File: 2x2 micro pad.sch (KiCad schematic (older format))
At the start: 24 parts, among them SW1 SW_Push, U1 ATmega32U4-AU, Y1 16MHz

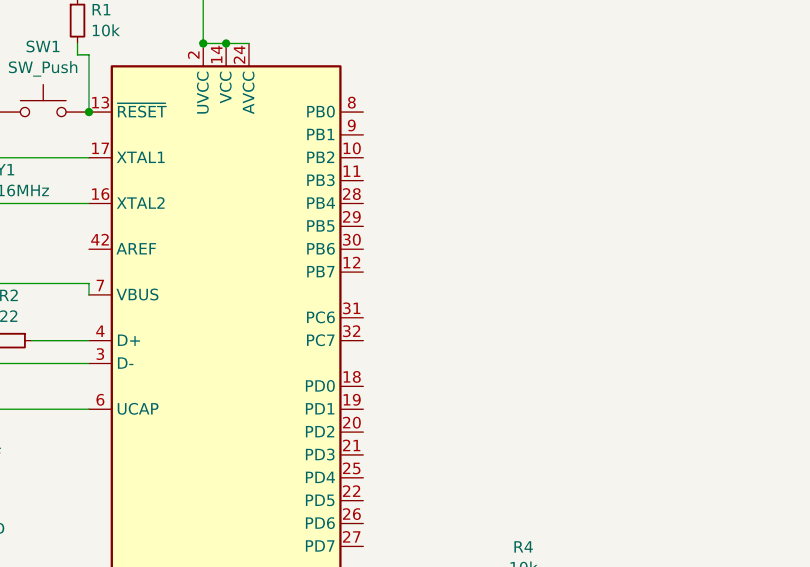
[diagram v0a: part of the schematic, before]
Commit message: pcb routing
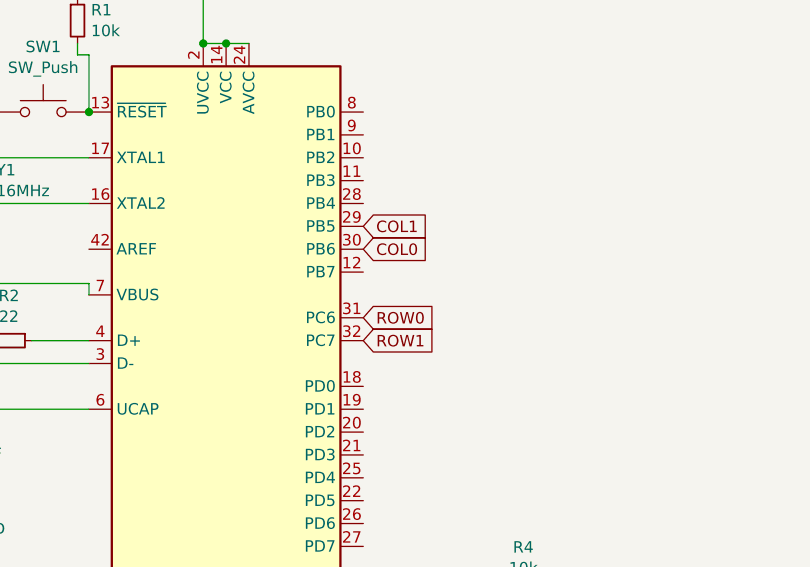
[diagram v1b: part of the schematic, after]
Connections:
- net COL0: now also U1.30 (PB6)
- net COL1: now also U1.29 (PB5)
- net ROW0: now also U1.31 (PC6)
- net ROW1: now also U1.32 (PC7)
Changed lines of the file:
@@
 EESchema Schematic File Version 4
+LIBS:2x2 micro pad-cache
 EELAYER 30 0
 EELAYER END
@@
 Text GLabel 6700 4100 0    50   Input ~ 0
 ROW1
+Text GLabel 4000 1950 2    50   Input ~ 0
+COL1
+Text GLabel 4000 2050 2    50   Input ~ 0
+COL0
+Text GLabel 4000 2350 2    50   Input ~ 0
+ROW0
+Text GLabel 4000 2450 2    50   Input ~ 0
+ROW1
 $EndSCHEMATC
